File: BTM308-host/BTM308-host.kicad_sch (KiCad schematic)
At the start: 45 parts, among them J1 Audio OUT, J2 USB_C_Receptacle_USB2.0_16P, J3 Battery Connector, SW1 PLAY, SW2 VOL+, SW3 VOL-, SW4 ON/OFF, U1 Bluetooth Module, U2 OPA1678

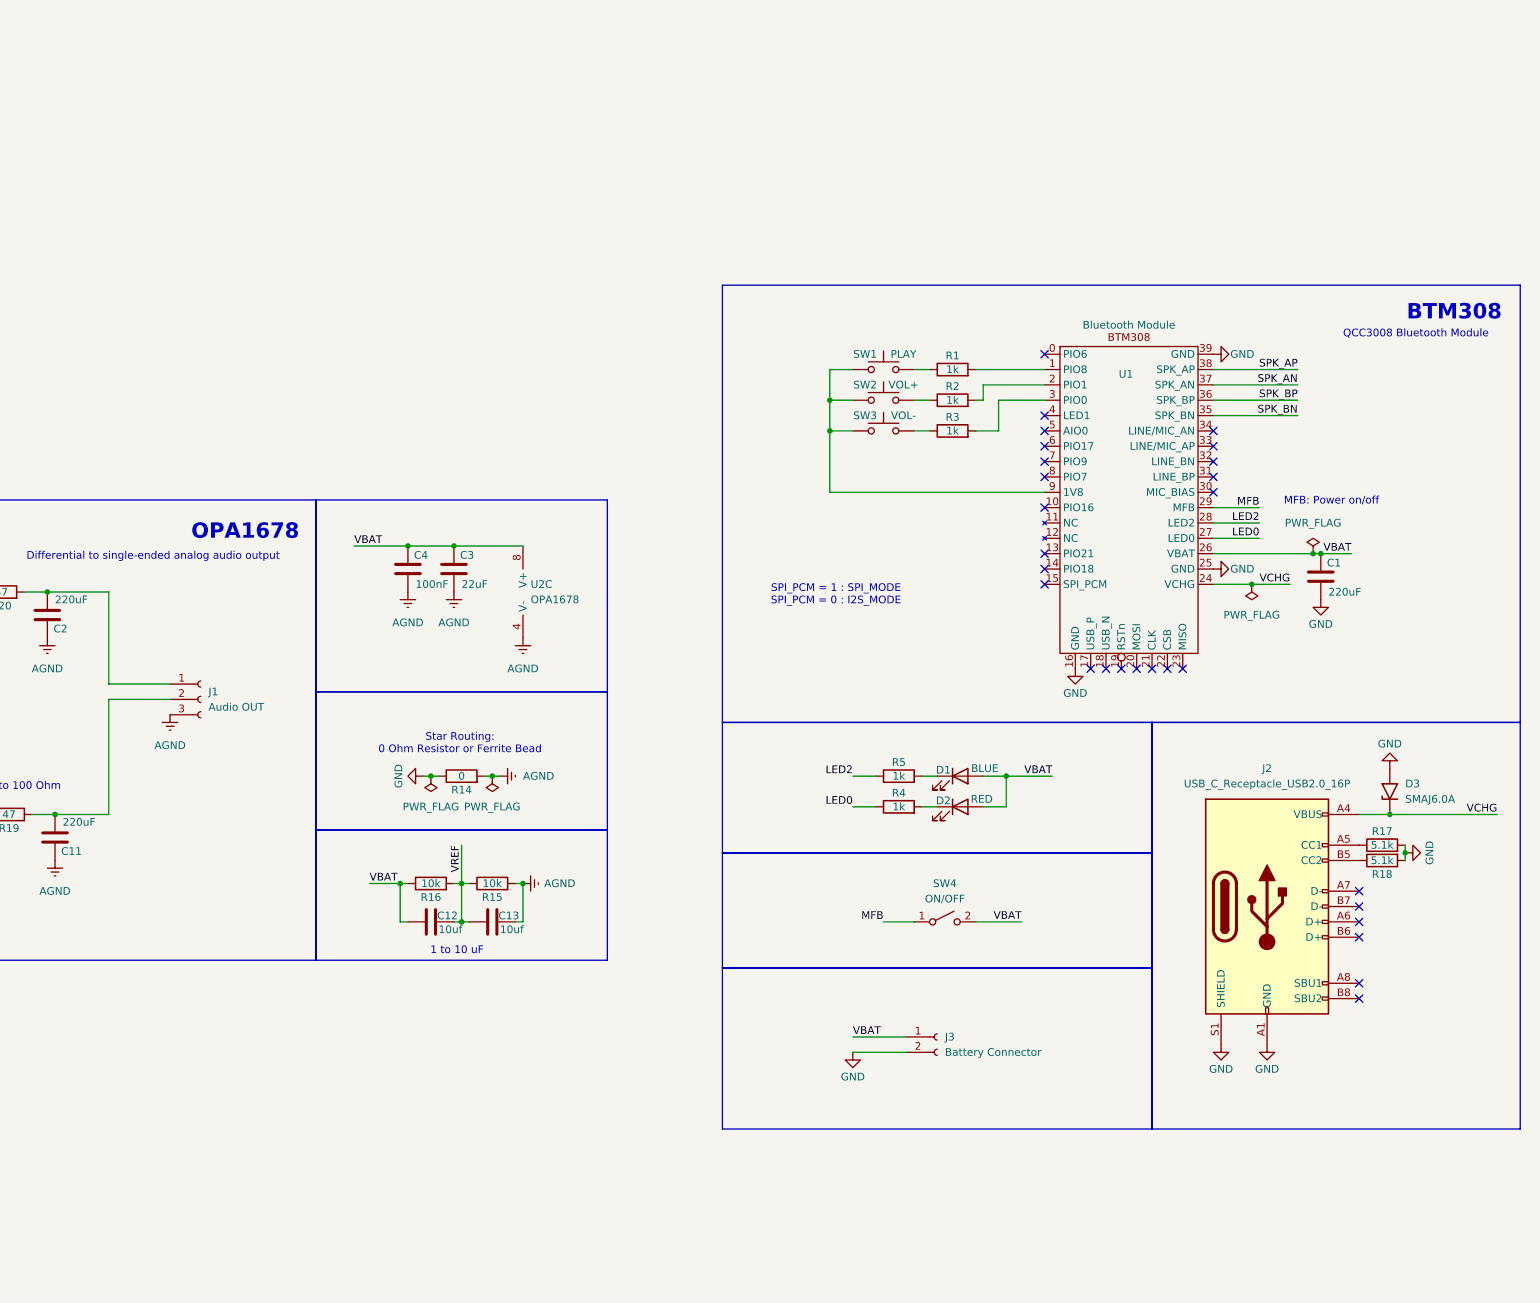
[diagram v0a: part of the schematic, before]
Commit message: layout position set
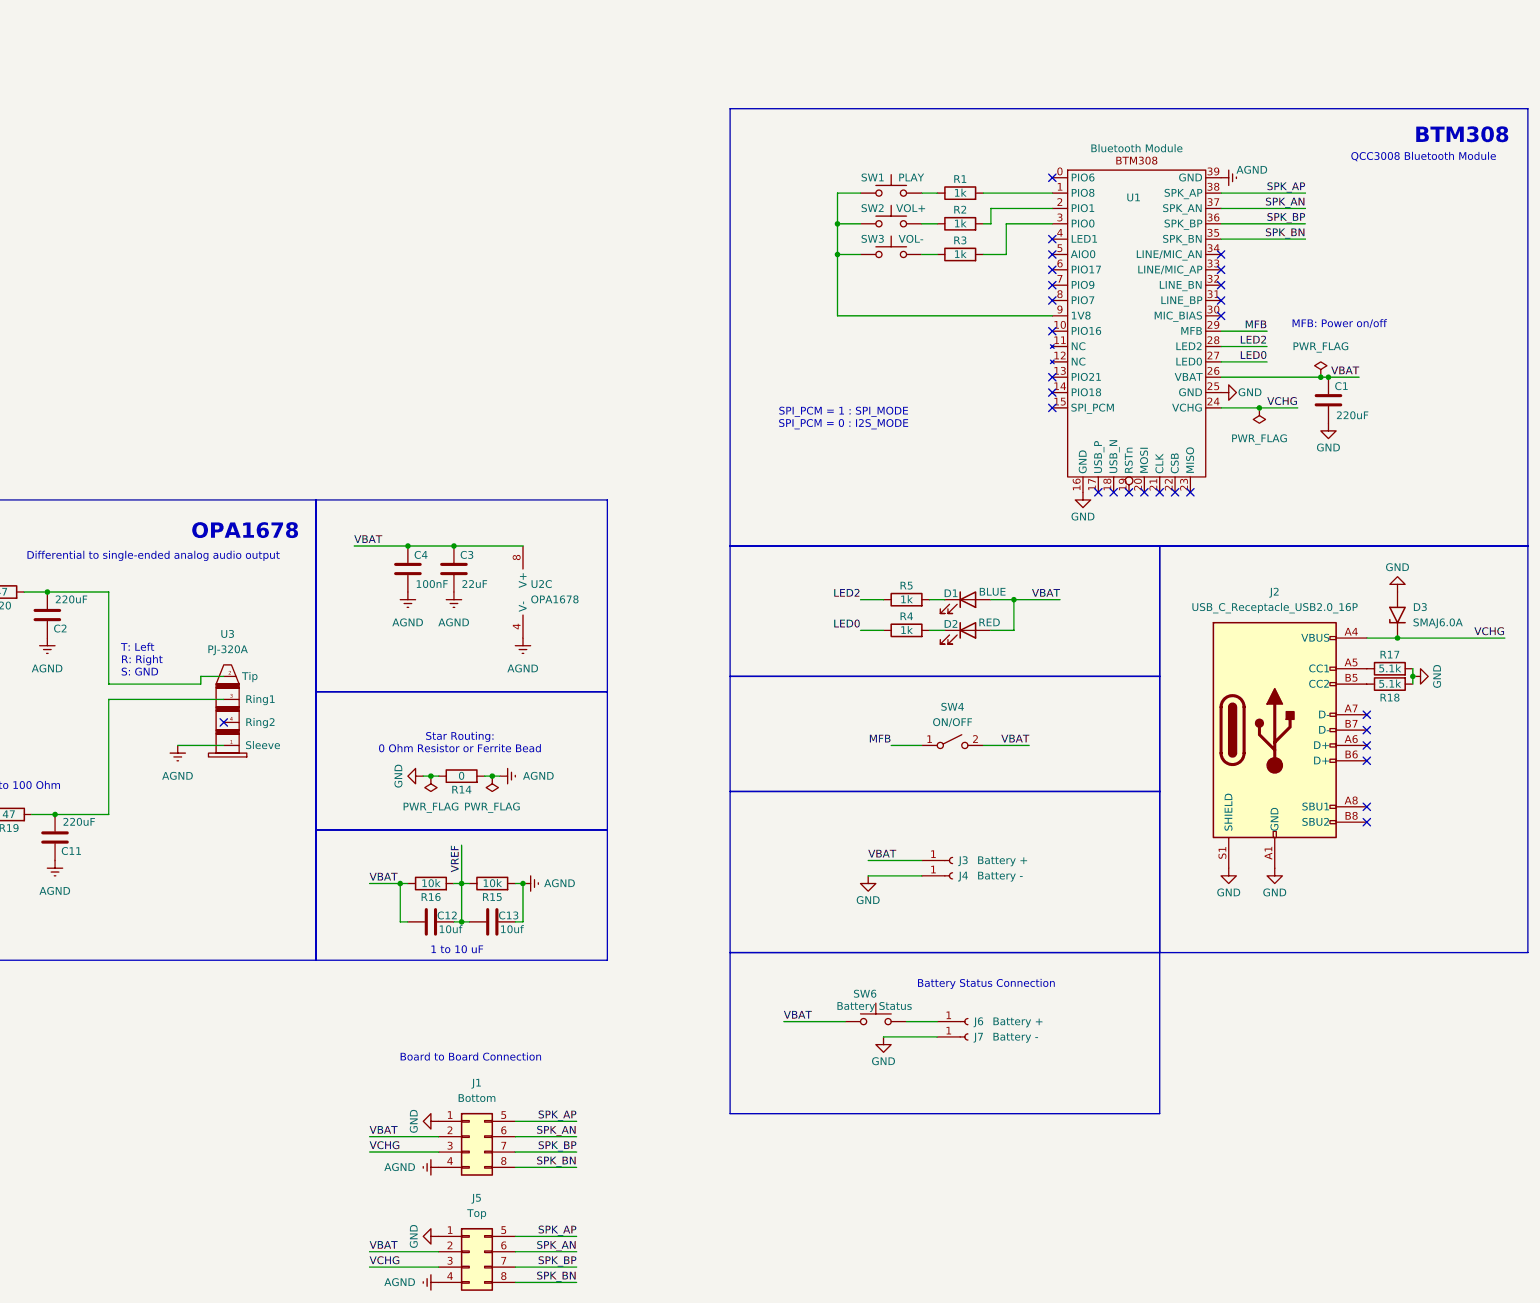
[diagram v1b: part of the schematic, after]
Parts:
- removed J1: Audio OUT, Connector_PinHeader_2.54mm:PinHeader_1x03_P2.54mm_Vertical, symbol Connector:Conn_01x03_Socket
- removed J3: Battery Connector, Connector_JST:JST_XH_S2B-XH-A_1x02_P2.50mm_Horizontal, symbol Connector:Conn_01x02_Socket
- added J1: Bottom, Connector_PinSocket_2.54mm:PinSocket_2x04_P2.54mm_Vertical, symbol Connector_Generic:Conn_02x04_Top_Bottom
- added J3, J6: Battery +, Connector_PinHeader_2.54mm:PinHeader_1x01_P2.54mm_Vertical, symbol Connector:Conn_01x01_Socket
- added J4, J7: Battery -, Connector_PinHeader_2.54mm:PinHeader_1x01_P2.54mm_Vertical, symbol Connector:Conn_01x01_Socket
- added J5: Top, Connector_PinHeader_2.54mm:PinHeader_2x04_P2.54mm_Vertical, symbol Connector_Generic:Conn_02x04_Top_Bottom
- added SW6: Battery Status, TS-A002:TST-A002_0.6MM_BOSS, symbol Switch:SW_Push
- added U3: PJ-320A, PJ-320A_Library:PJ-320A, symbol PJ-320A_Library:PJ-320A
- SW1, SW2, SW3: footprint (none) -> TS-A002:TST-A002_0.6MM_BOSS
- SW4: footprint (none) -> KiCad:SLW8645745ARAND
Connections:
- net AGND: now also U1.39 (GND), J1.4 (Pin_4), J5.4 (Pin_4), U3.1 (Sleeve)
- net GND: now also J1.1 (Pin_1), J4.1 (Pin_1), J5.1 (Pin_1), J7.1 (Pin_1); no longer U1.39 (GND)
- net SPK_AN: now also J1.6 (Pin_6), J5.6 (Pin_6)
- net SPK_AP: now also J1.5 (Pin_5), J5.5 (Pin_5)
- net SPK_BN: now also J1.8 (Pin_8), J5.8 (Pin_8)
- net SPK_BP: now also J1.7 (Pin_7), J5.7 (Pin_7)
- net VBAT: now also J1.2 (Pin_2), J3.1 (Pin_1), J5.2 (Pin_2), SW6.1
- net VCHG: now also J1.3 (Pin_3), J5.3 (Pin_3)
- net at C11.2, R19.2: now also U3.3 (Ring1)
- net at C2.2, R20.2: now also U3.2 (Tip)
- new net: J6.1 (Pin_1), SW6.2
- no-connect marks 28 -> 29
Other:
- note added: "Battery Status Connection"
- note added: "Board to Board Connection"
- note added: "T: Left R: Right S: GND"
- moved on the sheet: C1, D1, D2, D3, J2, R1, R17, R18, R2, R3, R4, R5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
